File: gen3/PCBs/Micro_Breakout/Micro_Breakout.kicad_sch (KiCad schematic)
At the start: 49 parts, among them J1 BlueRobotics Depth Sensor, J10 Kill Switch, J11 StarOddi CTD Comms, J12 LED1, J13 LED2, J14 Leak Sensor, J15 Extra I2C #3, J16 Extra I2C #6, J17 Extra I2C #5, J18 Extra I2C #4, J19 GND Line, J2 Interconnect, J20 3.3V Line, J21 5V Line, J22 Extra SPI #1, J23 Extra SPI #2, J24 Extra SPI #3, J25 Secondary UART, J3 External Battery, J4 Conn_01x24, J5 External I2C, J6 Conn_01x24, J7 Extra I2C #1, J8 Extra I2C #2, J9 Lumen PWM, Q7 L78M05ABDT-TR, U1 SHT31-DIS-B, U3 MS560702BA03-50, U4 AMS1117-3_3V_C5120796, U5 MCP9808-E_MS, U6 Teensy4_1

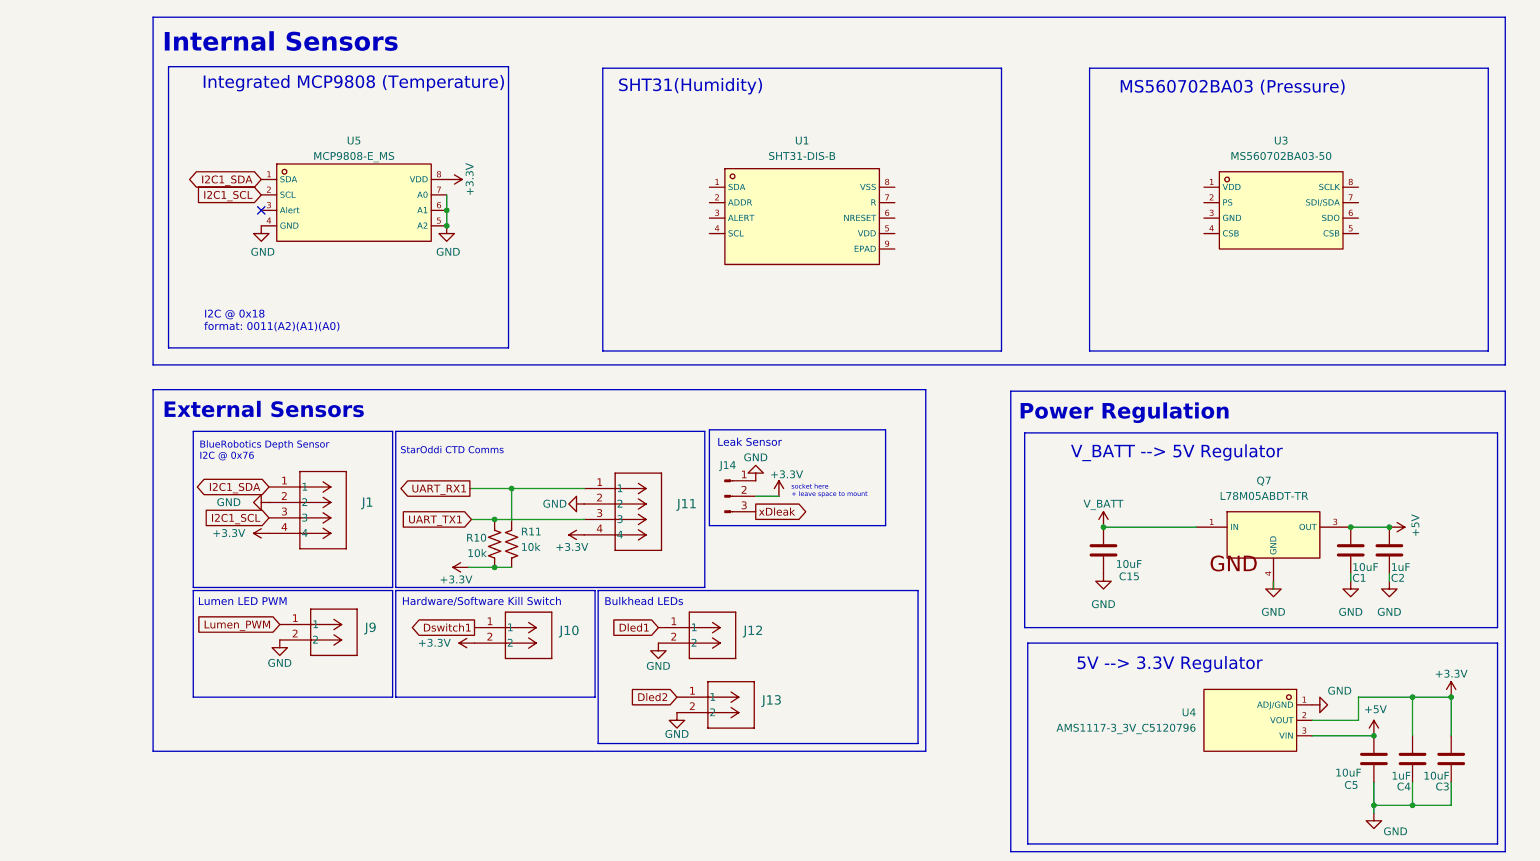
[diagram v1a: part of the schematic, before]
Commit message: wired correctly gen3 sub
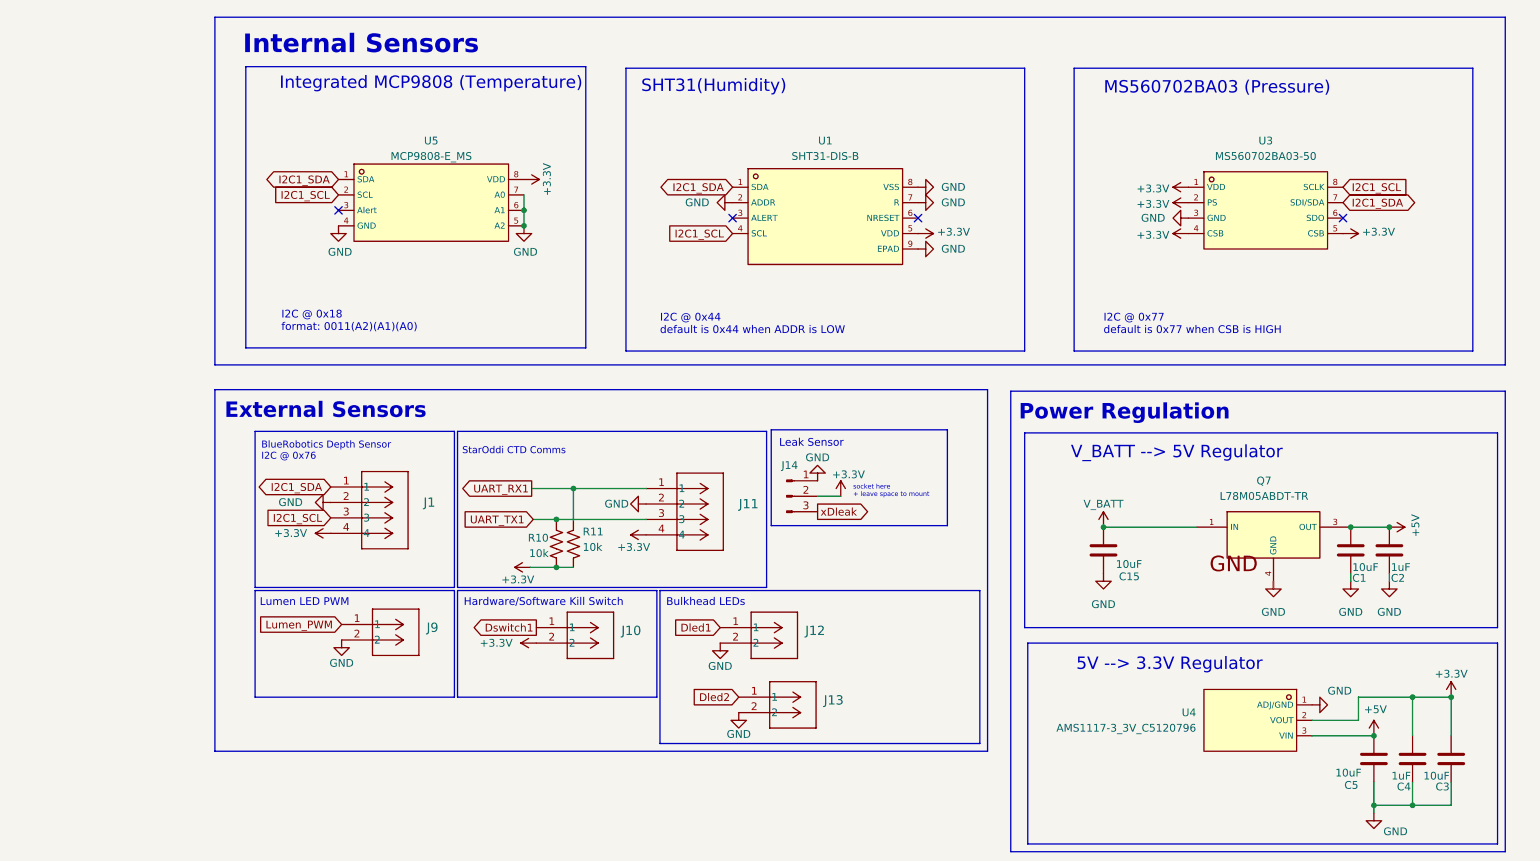
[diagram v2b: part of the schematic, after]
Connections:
- net +3.3V: now also U1.5 (VDD), U3.1 (VDD), U3.2 (PS), U3.4 (CSB), U3.5 (CSB)
- net GND: now also U1.2 (ADDR), U1.7 (R), U1.8 (VSS), U1.9 (EPAD), U3.3 (GND)
- net I2C1_SCL: now also U1.4 (SCL), U3.8 (SCLK)
- net I2C1_SDA: now also U1.1 (SDA), U3.7 (SDI/SDA)
- no-connect marks 25 -> 28
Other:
- note added: "I2C @ 0x44 default is 0x44 when ADDR is LOW"
- note added: "I2C @ 0x77 default is 0x77 when CSB is HIGH"
- moved on the sheet: J1, J10, J11, J12, J13, J14, J9, R10, R11, U1, U3, U5
